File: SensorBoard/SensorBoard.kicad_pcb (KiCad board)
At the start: 2 copper layers, 25 x 15.5 mm, 13 parts, among them J1 to MAIN, Q1 2SC2712-Y, Q2 2SC2712-Y, Q3 2SC2712-Y

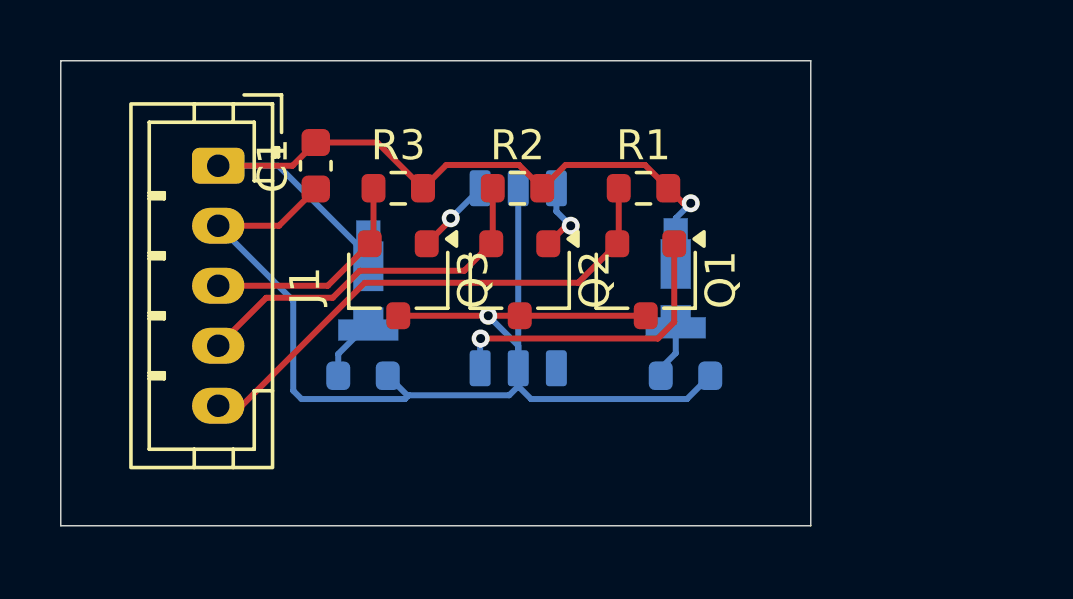
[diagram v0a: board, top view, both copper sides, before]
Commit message: パターン終了
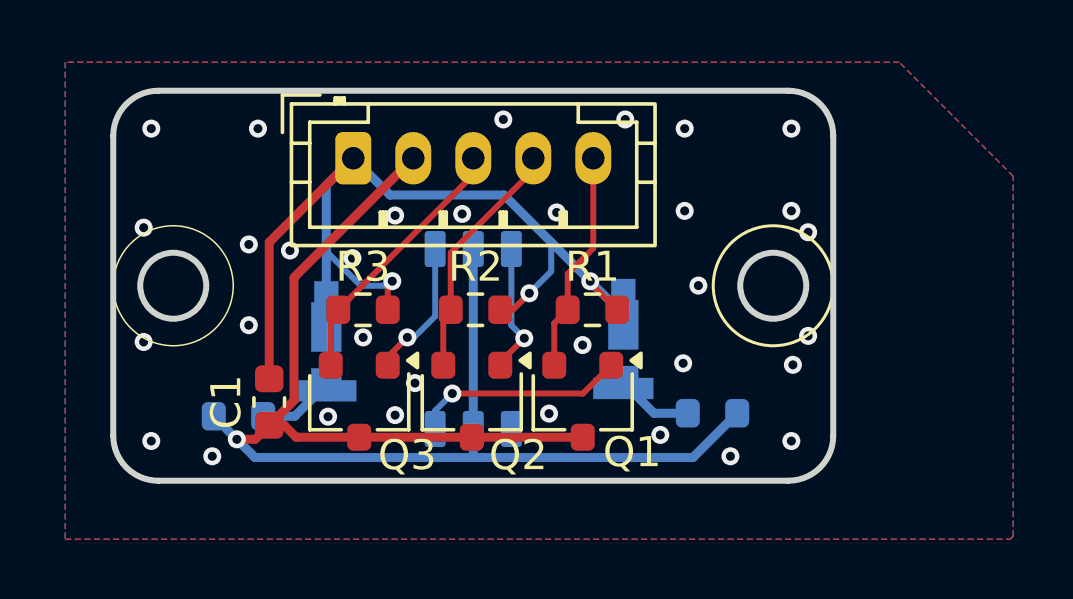
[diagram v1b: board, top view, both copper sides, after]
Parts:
- moved C1 8.03 mm to (52.7, 41.6)
- moved Q1 4.56 mm to (63.1, 41.6)
- moved J1 4.51 mm to (55.5, 33.5), turned to 0 degrees
- moved R1 4.39 mm to (63.5, 38.5)
- moved R4 4.36 mm to (51.7, 42.1), turned to 0 degrees
- moved Q2 4.35 mm to (59.5, 41.6)
- moved R2 4.29 mm to (59.6, 38.5)
- moved Q3 4.25 mm to (55.7, 41.6)
- moved R3 4.22 mm to (55.8, 38.5)
- moved D2 2.68 mm to (64.5, 39.5)
- moved S1 2.52 mm to (59.5, 39.5)
- moved D1 2.46 mm to (54.6, 39.6)
- moved R5 1.54 mm to (67.5, 42.0)
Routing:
- net /S_B: track 17.4 -> 7.44 mm
- net GND: track 26.4 -> 33.6 mm, vias 1 -> 36
- net +3V3: track 43.0 -> 48.4 mm
- net /S_G: track 12.4 -> 8.14 mm
- net /Blue: track 10.3 -> 7.11 mm
- net /Red: track 2.59 -> 4.66 mm
- net /Green: track 2.45 -> 4.38 mm
- net /S_R: track 7.53 -> 8.87 mm
- net Net-(D2-PadA): track 2.01 -> 2.57 mm
- added copper zone on B.Cu, net GND
- added copper zone on F.Cu, net GND
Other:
- board size 25 x 15.5 mm -> 24 x 13 mm
